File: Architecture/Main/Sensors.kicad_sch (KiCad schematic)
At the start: 0 parts

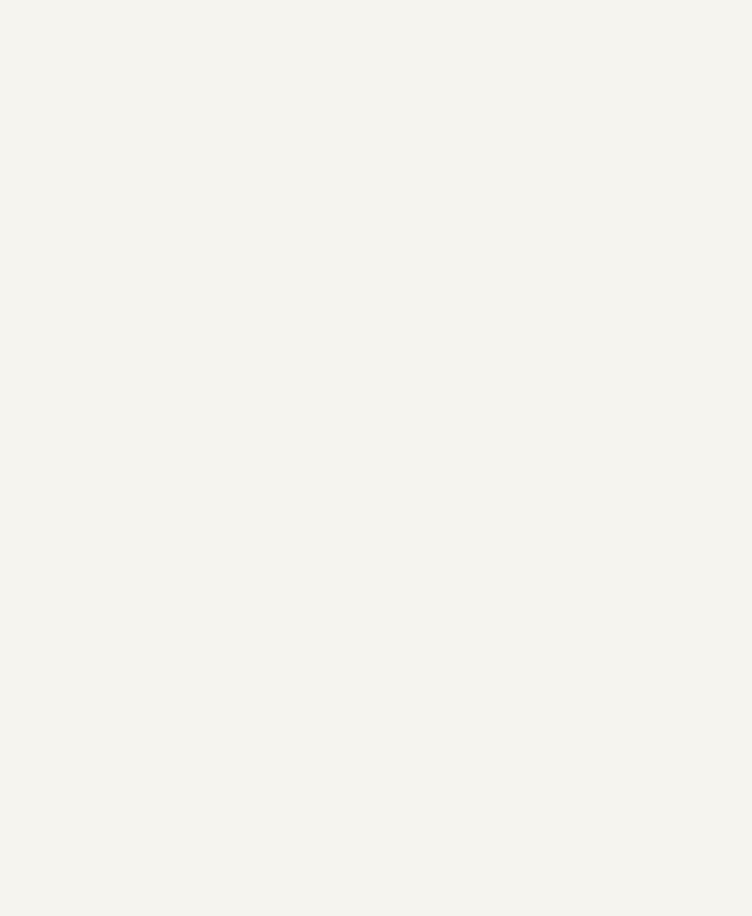
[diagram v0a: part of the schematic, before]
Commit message: Archi_1
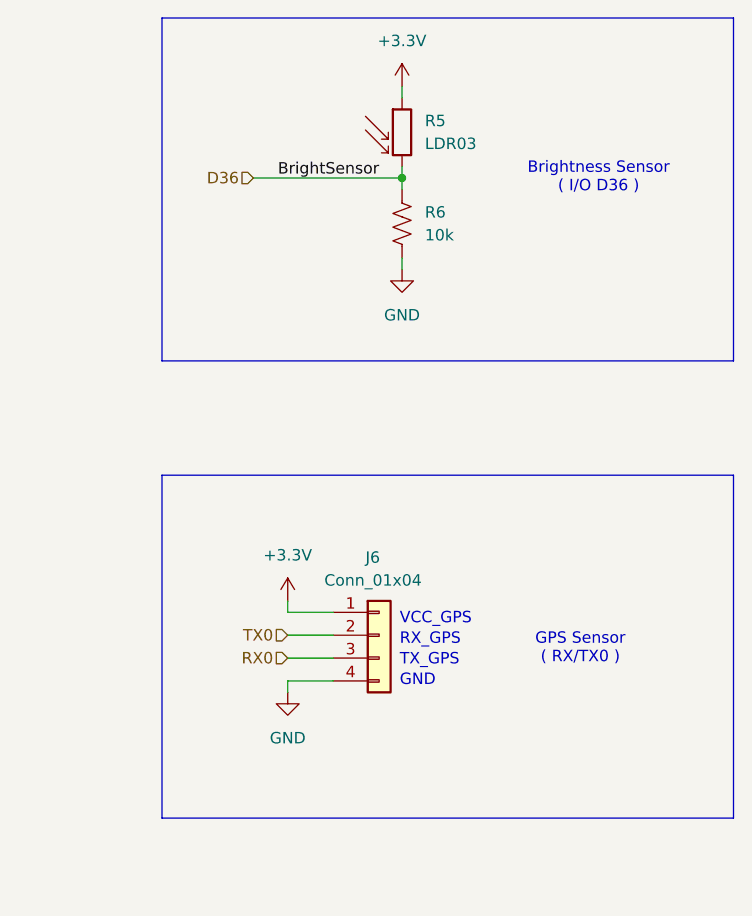
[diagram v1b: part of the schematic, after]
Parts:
- added J6: Conn_01x04, symbol Connector_Generic:Conn_01x04
- added R5: LDR03, OptoDevice:R_LDR_10x8.5mm_P7.6mm_Vertical, symbol Sensor_Optical:LDR03
- added R6: 10k, symbol Device:R_US
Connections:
- net +3.3V: now also J6.1 (Pin_1), R5.1
- net GND: now also J6.4 (Pin_4), R6.2
- new net D36: R5.2, R6.1
- new net RX0: J6.3 (Pin_3)
- new net TX0: J6.2 (Pin_2)
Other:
- note added: "Brightness Sensor ( I/O D36 )"
- note added: "GND"
- note added: "GPS Sensor ( RX/TX0 )"
- note added: "RX_GPS"
- note added: "TX_GPS"
- note added: "VCC_GPS"
